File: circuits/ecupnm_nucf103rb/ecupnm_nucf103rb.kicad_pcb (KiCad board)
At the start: 2 copper layers, 70.6 x 64.8 mm, 41 parts, among them J1 Conn_01x02_Pin, J2 Conn_01x02_Pin, J3 Conn_01x03_Pin, J4 USB_B_Mini, Q1 2N3904, Q2 IRF540N, Q3 IRF540N, U1 NUCLEO-64, U2 H11L1, U3 AMS1117-5.0, U4 4N35, U5 FT232RL, U6 4N35

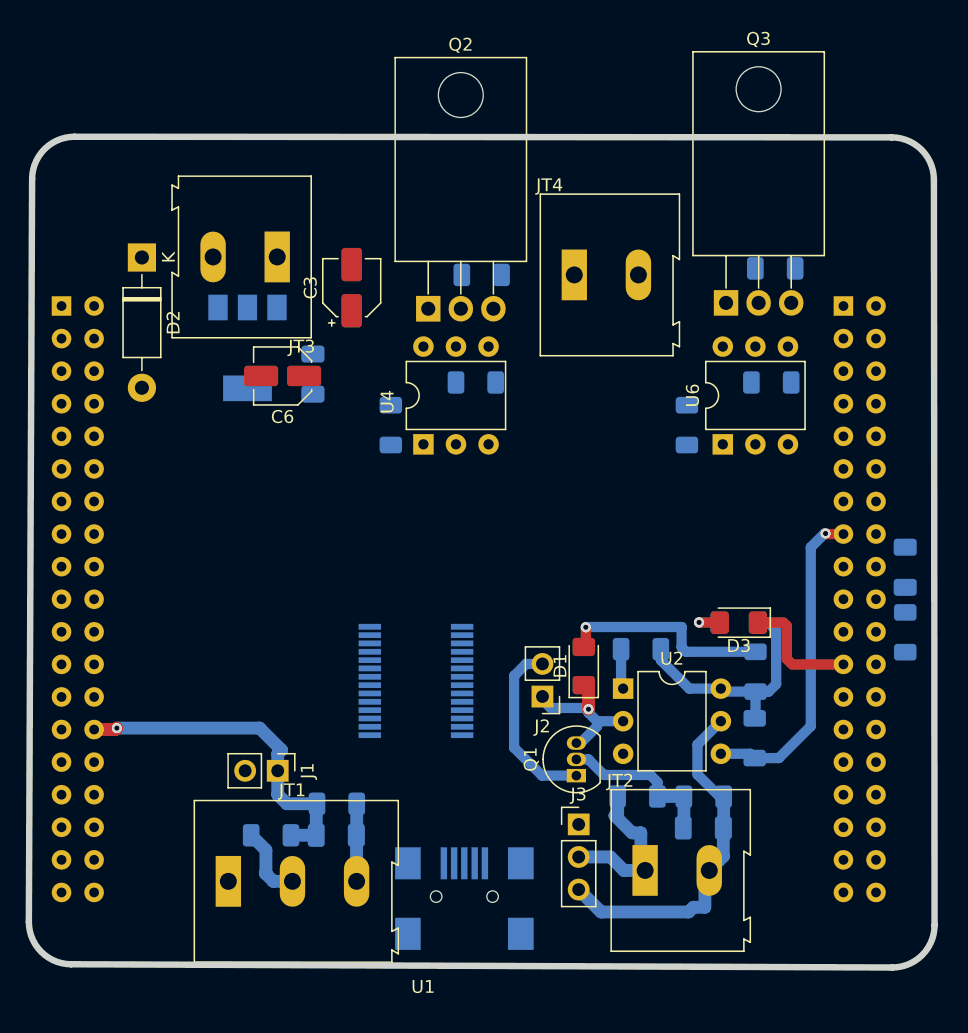
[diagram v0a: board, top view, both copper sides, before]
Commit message: Nucleo Based
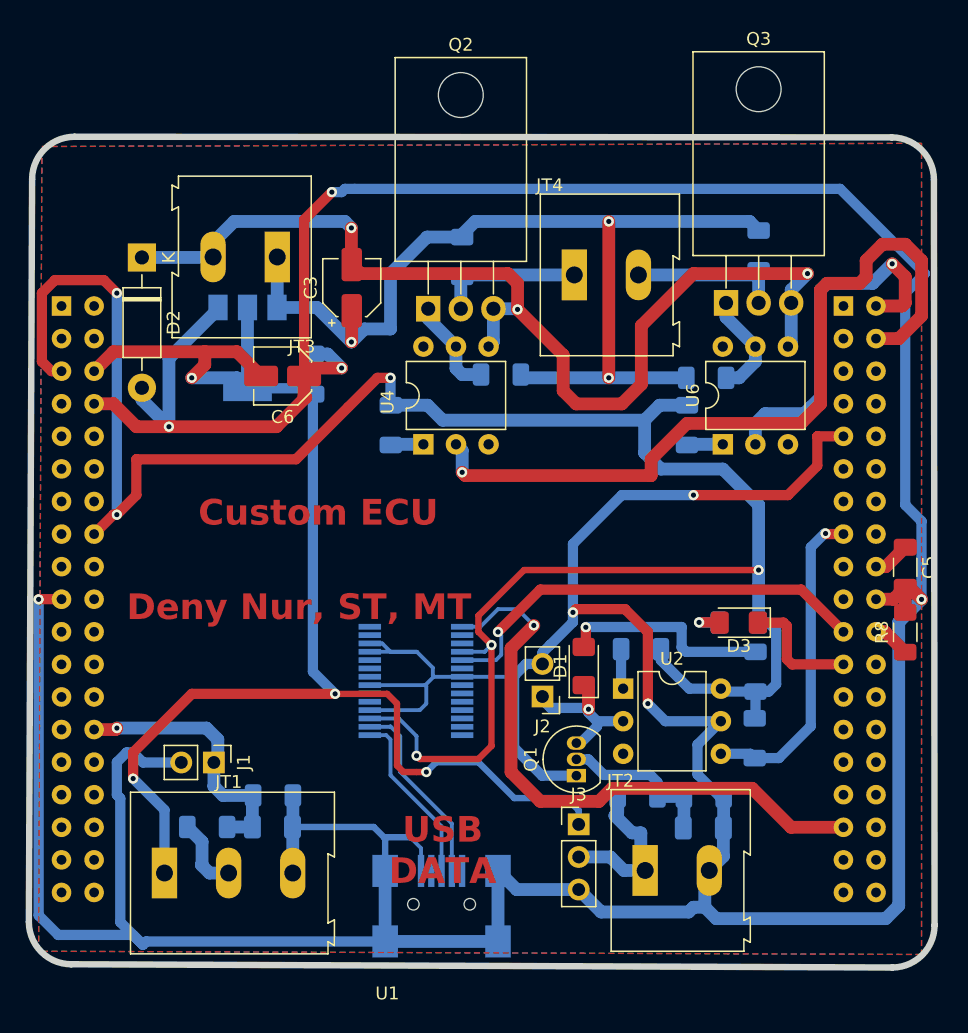
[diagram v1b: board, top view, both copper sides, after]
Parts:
- C5, R8: moved to F.Cu
- moved R14 5.09 mm to (147.3, 77.7), turned to 0 degrees
- moved JT1 5.02 mm to (105.1, 116.3)
- moved R1 5.02 mm to (108.4, 112.7)
- moved R2 5.02 mm to (113.5, 110.3)
- moved C1 5.02 mm to (113.5, 112.7)
- moved J1 5.02 mm to (108.9, 107.7)
- moved R12 2.07 mm to (128.3, 68.3), turned to -90 degrees
- moved R11 2.05 mm to (131.3, 77.5)
- moved R15 1.91 mm to (151.4, 67.8), turned to -90 degrees
- moved J4 1.88 mm to (126.7, 118.8)
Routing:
- net GND: track 47.6 -> 425.5 mm, vias 0 -> 8
- net VDD: track 19.0 -> 176.9 mm, vias 0 -> 6
- net VCC: track 0.00 -> 115.3 mm, vias 0 -> 4
- net GNDPWR: track 0.00 -> 82.3 mm, vias 0 -> 3
- net +12V: track 0.00 -> 77.1 mm, vias 0 -> 3
- net OUT_INJ: track 0.00 -> 61.6 mm, vias 0 -> 1
- net RX: track 0.00 -> 47.4 mm, vias 0 -> 1
- net TX: track 0.00 -> 34.8 mm, vias 0 -> 1
- net OUT_IGN: track 0.00 -> 28.2 mm, vias 0 -> 1
- net Net-(J4-D-): track 0.00 -> 14.9 mm
- net Net-(J4-D+): track 0.00 -> 13.6 mm
- net PORT_IGN: track 0.00 -> 12.1 mm
- net PORT_INJ: track 0.00 -> 11.3 mm
- net Net-(Q3-G): track 0.00 -> 8.33 mm
- net Net-(Q2-G): track 0.00 -> 7.70 mm
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- added copper zone on B.Cu, net (none)
- added copper zone on F.Cu, net (none)
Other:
- board text added: "Custom ECU"
- board text added: "Deny Nur, ST, MT"
- board text added: "USB DATA"
